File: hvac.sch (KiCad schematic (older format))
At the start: 51 parts, among them IC1 ATMEGA328P-A, J1 PROGRAMMING HEADER, J2 SERIAL PORT, J3 POWER_INPUT, M1 FIDUCIAL, M2 FIDUCIAL, M3 FIDUCIAL, SW1 SPST, SW2 SPST, SW3 SPST, U1 MIC5225, U2 MOSFET_N, U3 MOSFET_N, U4 MOSFET_N

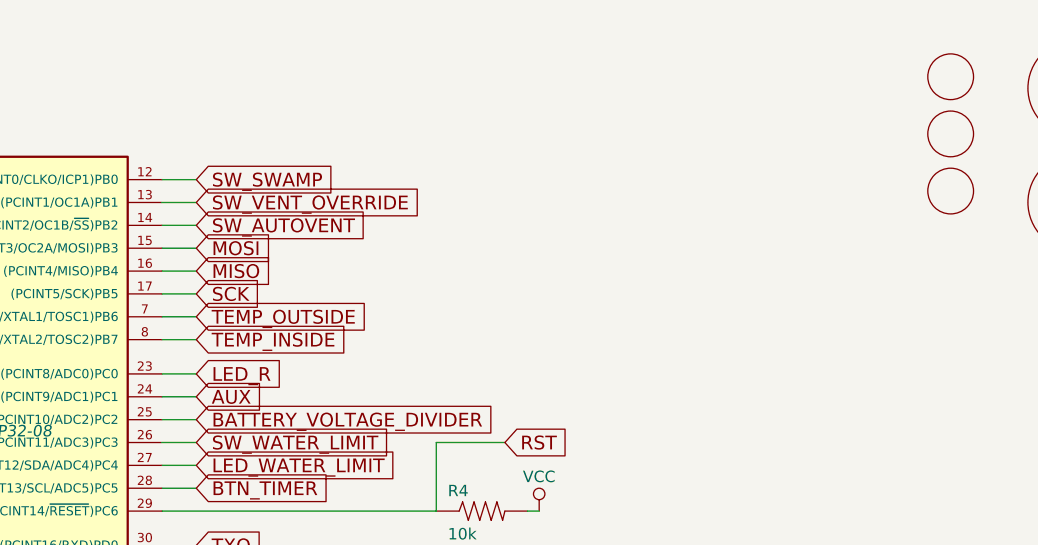
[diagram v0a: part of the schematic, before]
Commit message: Move pieces to fit better
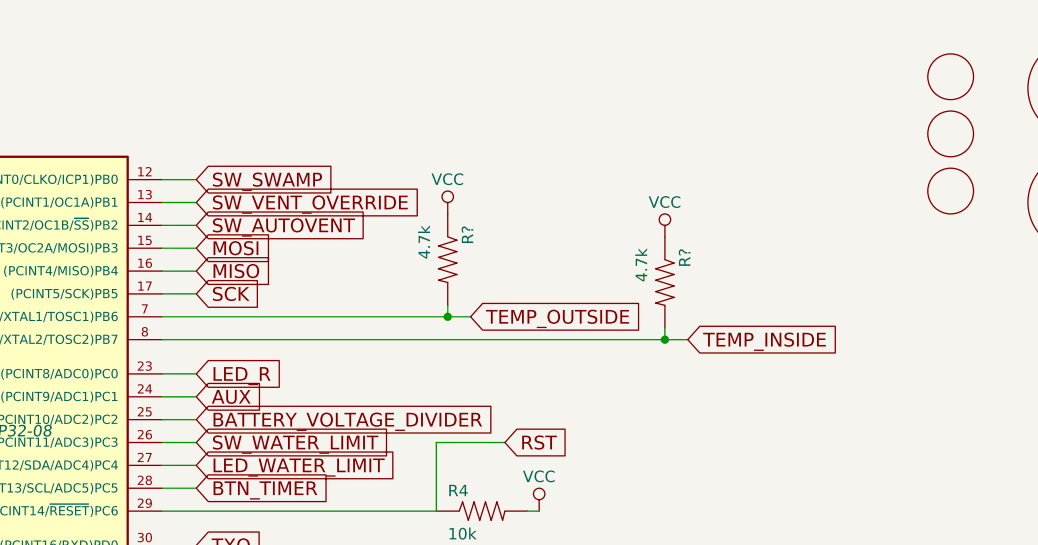
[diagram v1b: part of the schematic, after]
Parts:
- added R? (x2): 4.7k, 0402-RES, symbol RESISTOR0402
- BTN1: footprint homebrew:EG2355-ND -> homebrew:PVA1-OA-H2
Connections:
- net TEMP_INSIDE: now also R?.2
- net TEMP_OUTSIDE: now also R?.2
- net VCC: now also R?.1, R?.1
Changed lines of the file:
@@
 Wire Wire Line
 	3850 2800 4000 2800
-Text GLabel 4000 1800 2    60   Input ~ 0
+Text GLabel 5200 1800 2    60   Input ~ 0
 TEMP_OUTSIDE
-Text GLabel 4000 1900 2    60   Input ~ 0
+Text GLabel 6150 1900 2    60   Input ~ 0
 TEMP_INSIDE
 Wire Wire Line
-	4000 1900 3850 1900
-Wire Wire Line
-	3850 1800 4000 1800
+	3850 1900 6150 1900
+Wire Wire Line
+	3850 1800 5200 1800
 Wire Wire Line
 	3850 2650 5050 2650
@@
 F 0 "BTN1" H 9500 1550 50  0000 C CNN
 F 1 "SPST" H 9500 1350 50  0001 C CNN
-F 2 "homebrew:EG2355-ND" H 9500 1450 50  0001 C CNN
+F 2 "homebrew:PVA1-OA-H2" H 9500 1450 50  0001 C CNN
 F 3 "" H 9500 1450 50  0000 C CNN
 	1    9500 1450
@@
 	1    0    0    -1
 $EndComp
+$Comp
+L RESISTOR0402 R?
+U 1 1 5965B0E5
+P 6050 1650
+F 0 "R?" H 5900 1709 50  0000 L BNN
+F 1 "4.7k" H 5900 1520 50  0000 L BNN
+F 2 "0402-RES" H 6080 1800 20  0001 C CNN
+F 3 "" H 6050 1650 60  0000 C CNN
+	1    6050 1650
+	0    1    1    0
+$EndComp
+$Comp
+L RESISTOR0402 R?
+U 1 1 5965B1A0
+P 5100 1550
+F 0 "R?" H 4950 1609 50  0000 L BNN
+F 1 "4.7k" H 4950 1420 50  0000 L BNN
+F 2 "0402-RES" H 5130 1700 20  0001 C CNN
+F 3 "" H 5100 1550 60  0000 C CNN
+	1    5100 1550
+	0    1    1    0
+$EndComp
+Wire Wire Line
+	5100 1750 5100 1800
+Connection ~ 5100 1800
+Wire Wire Line
+	6050 1900 6050 1850
+Connection ~ 6050 1900
+$Comp
+L VCC #PWR?
+U 1 1 5965C4CF
+P 5100 1350
+F 0 "#PWR?" H 5100 1200 50  0001 C CNN
+F 1 "VCC" H 5100 1500 50  0000 C CNN
+F 2 "" H 5100 1350 50  0000 C CNN
+F 3 "" H 5100 1350 50  0000 C CNN
+	1    5100 1350
+	1    0    0    -1
+$EndComp
+$Comp
+L VCC #PWR?
+U 1 1 5965C60B
+P 6050 1450
+F 0 "#PWR?" H 6050 1300 50  0001 C CNN
+F 1 "VCC" H 6050 1600 50  0000 C CNN
+F 2 "" H 6050 1450 50  0000 C CNN
+F 3 "" H 6050 1450 50  0000 C CNN
+	1    6050 1450
+	1    0    0    -1
+$EndComp
